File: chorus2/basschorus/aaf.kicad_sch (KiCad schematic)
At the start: 12 parts, among them U2 TL074

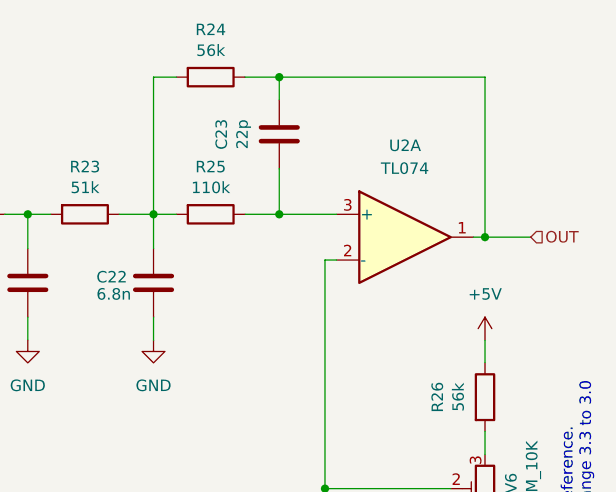
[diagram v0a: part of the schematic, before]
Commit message: basic layout
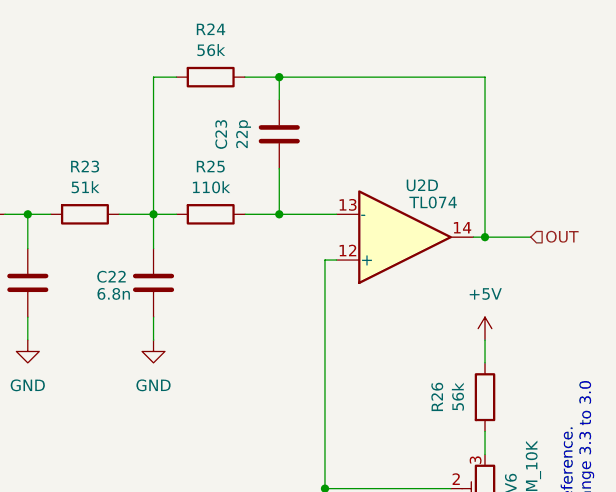
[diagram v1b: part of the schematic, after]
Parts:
- removed U2: TL074, Package_SO:SO-14_3.9x8.65mm_P1.27mm, symbol Amplifier_Operational:TL074
- added U2: TL074, Package_SO:SO-14_3.9x8.65mm_P1.27mm, symbol Amplifier_Operational:TL074
- R22, R23, R24, R25, R26, R27: footprint Resistor_THT:R_Axial_DIN0204_L3.6mm_D1.6mm_P5.08mm_Horizontal -> Resistor_THT:R_Axial_DIN0204_L3.6mm_D1.6mm_P2.54mm_Vertical
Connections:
- net OUT: now also U2.14
- net at RV6.2, TP1.1: now also U2.12 (+)
- net at C23.2, R25.1: now also U2.13 (-)
